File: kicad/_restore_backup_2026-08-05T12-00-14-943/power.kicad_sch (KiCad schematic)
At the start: 19 parts, among them J4 2.1mm ID 5.5mm OD PJ-102AH, Q1 DMP3013SFV, U10 TLV75733PDBV, U11 TLV75733PDBV, U9 TPS62163DSG

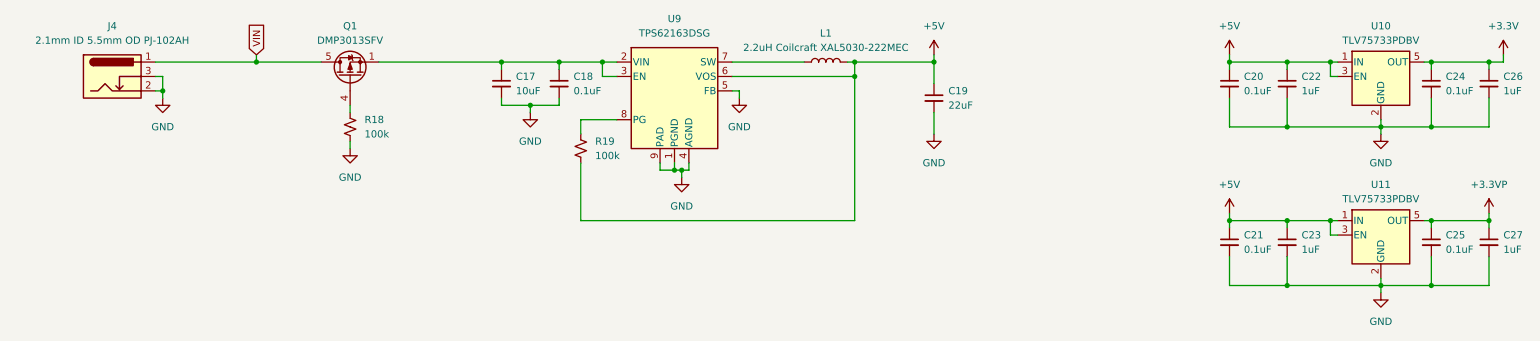
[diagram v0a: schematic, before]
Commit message: finish pcb
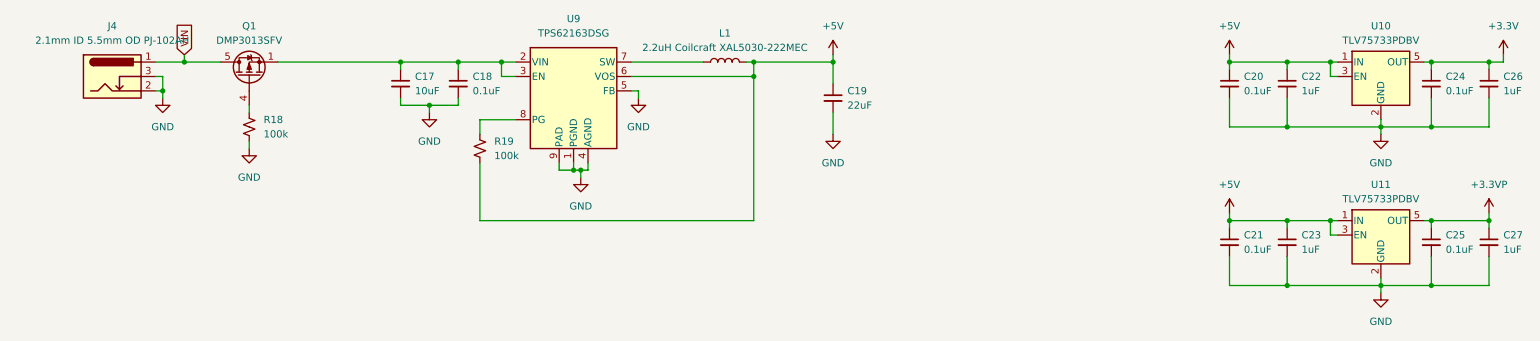
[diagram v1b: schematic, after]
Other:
- moved on the sheet: C17, C18, C19, L1, Q1, R18, R19, U9
